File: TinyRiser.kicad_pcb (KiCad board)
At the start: 4 copper layers, 113.2 x 23.5 mm, 32 parts, among them J2 Bus_PCI_Express_x16, J3 Bus_M.2_Socket_M, J4 fancontrol_header, M1 Fan_4pin

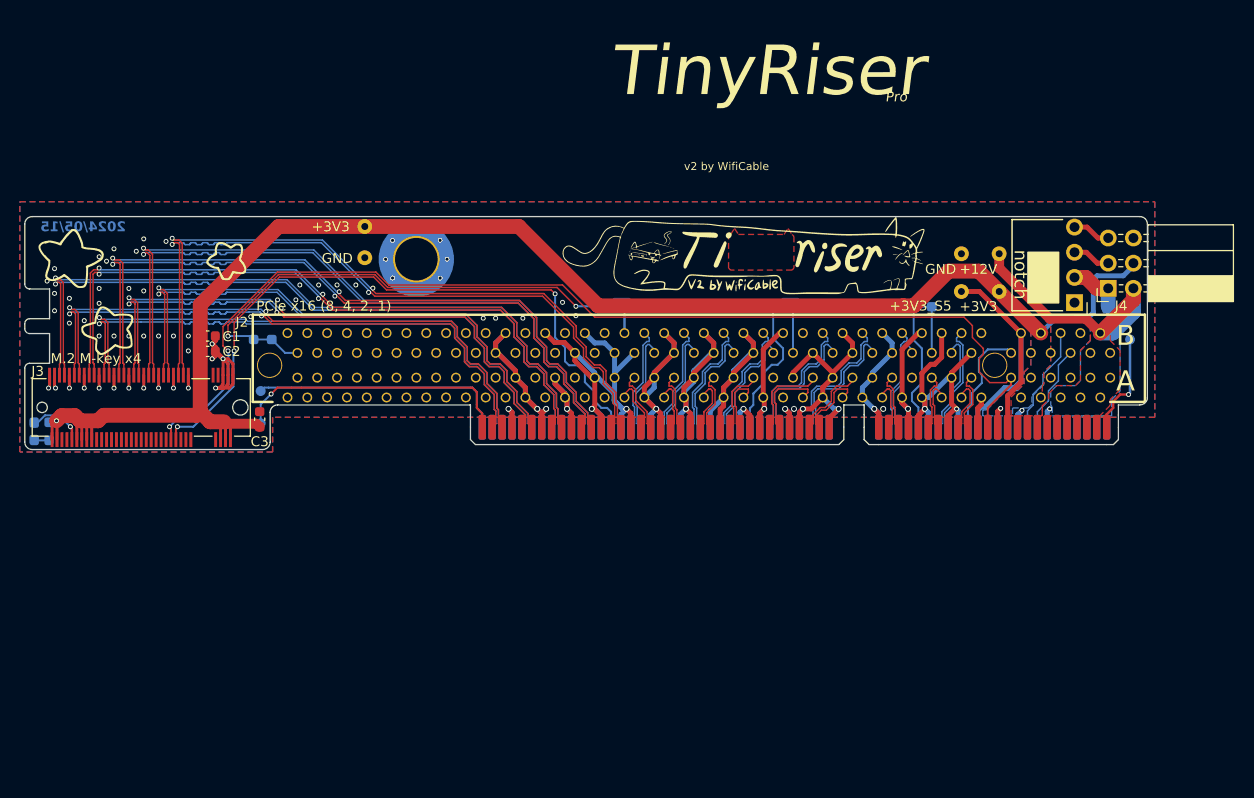
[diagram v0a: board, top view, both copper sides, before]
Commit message: long
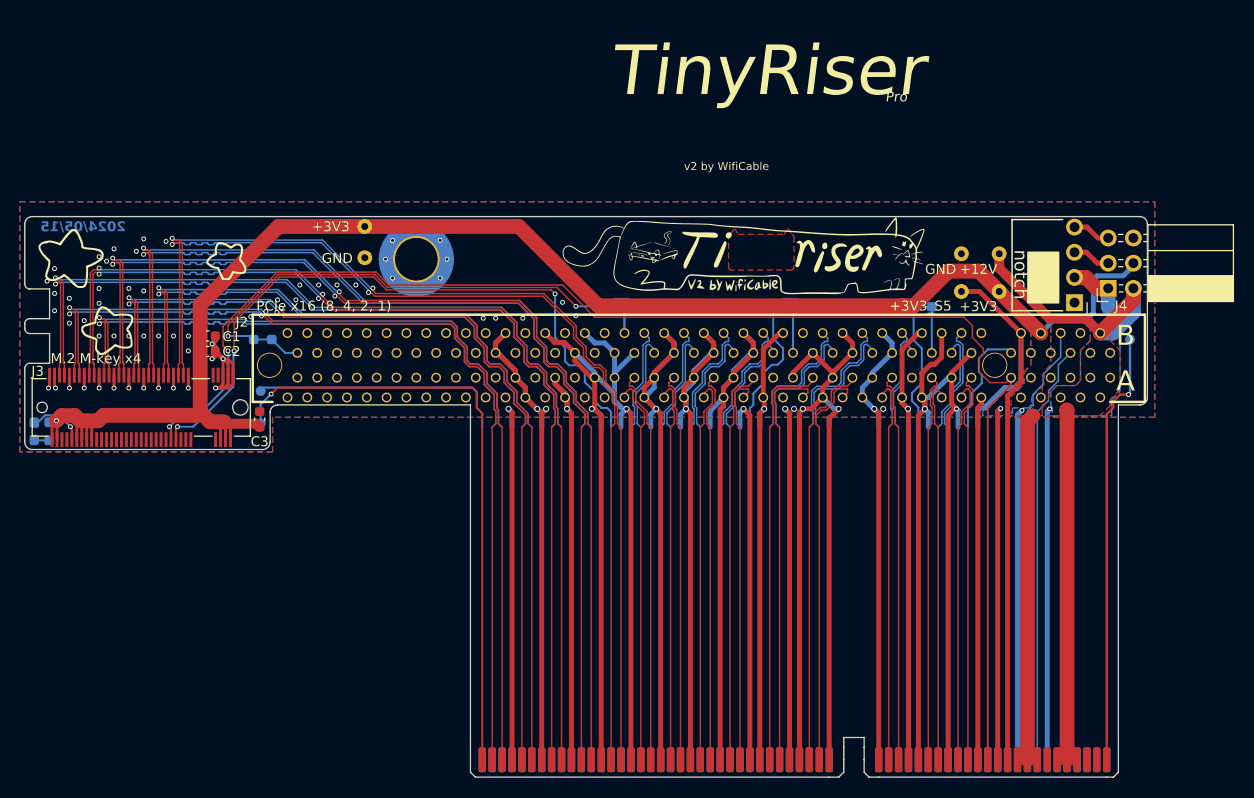
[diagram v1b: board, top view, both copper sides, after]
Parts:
- moved J1 33.6 mm to (123.2, 179.3)
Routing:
- net GND: track 296.7 -> 1001.3 mm
- net +12V: track 26.9 -> 62.2 mm
- net +3V3: track 158.7 -> 193.6 mm
- net PCIe_PCH_Tx1+: track 58.0 -> 91.5 mm
- net PCIe_CPU_REFCLK-: track 5.68 -> 39.2 mm
- net SMBDATA: track 10.9 -> 44.4 mm
- net PCIe_PCH_Tx1-: track 58.2 -> 91.7 mm
- net PCIe_PCH_Rx2-: track 68.9 -> 102.5 mm
- net PCIe_PCH_Rx2+: track 69.1 -> 102.6 mm
- net PCIe_PCH_Rx1-: track 72.0 -> 105.5 mm
- net PCIe_PCH_REFCLK+: track 71.6 -> 105.1 mm
- net PCIe_CPU_Rx7-: track 5.81 -> 39.4 mm
- net PCIe_CPU_Rx7+: track 6.27 -> 39.8 mm
- net PCIe_CPU_Rx6-: track 5.39 -> 38.9 mm
- net PCIe_CPU_Rx5-: track 5.67 -> 39.2 mm
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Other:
- board size 113.2 x 23.5 mm -> 113.2 x 52.6 mm

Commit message: unlong
definitely not shitposting in my git repo
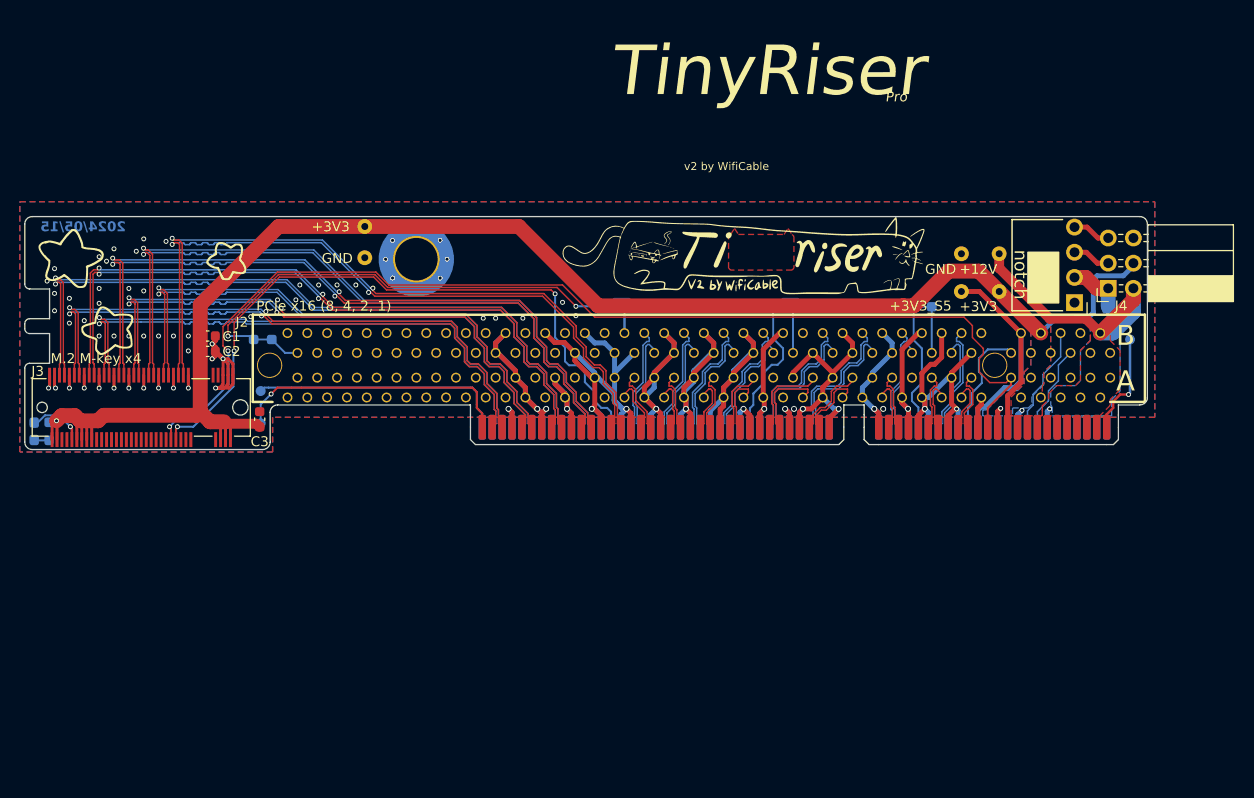
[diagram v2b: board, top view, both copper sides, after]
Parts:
- moved J1 33.6 mm to (123.2, 145.8)
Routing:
- net GND: track 1001.3 -> 296.7 mm
- net +12V: track 62.2 -> 26.9 mm
- net +3V3: track 193.6 -> 158.7 mm
- net PCIe_PCH_Tx1+: track 91.5 -> 58.0 mm
- net PCIe_CPU_REFCLK-: track 39.2 -> 5.68 mm
- net SMBDATA: track 44.4 -> 10.9 mm
- net PCIe_PCH_Tx1-: track 91.7 -> 58.2 mm
- net PCIe_PCH_Rx2-: track 102.5 -> 68.9 mm
- net PCIe_PCH_Rx2+: track 102.6 -> 69.1 mm
- net PCIe_PCH_Rx1-: track 105.5 -> 72.0 mm
- net PCIe_PCH_REFCLK+: track 105.1 -> 71.6 mm
- net PCIe_CPU_Rx7-: track 39.4 -> 5.81 mm
- net PCIe_CPU_Rx7+: track 39.8 -> 6.27 mm
- net PCIe_CPU_Rx6-: track 38.9 -> 5.39 mm
- net PCIe_CPU_Rx5-: track 39.2 -> 5.67 mm
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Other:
- board size 113.2 x 52.6 mm -> 113.2 x 23.5 mm
